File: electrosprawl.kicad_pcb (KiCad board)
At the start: 2 copper layers, 73.8 x 89.6 mm, 50 parts, among them J1 3.3v, J2 Conn_02x08_Counter_Clockwise, J3 Conn_02x06_Counter_Clockwise, J4 Conn_02x04_Counter_Clockwise, J5 Conn_02x08_Counter_Clockwise, J6 3.3v, J67 Conn_02x05_Counter_Clockwise, J7 VCC, J70 TXRX, J71 Micro_SD_Card_Det, J74 USB_B_Micro, SW1 Reset, U2 samd51p20, U5 LM1117-3.3, Y1 Crystal

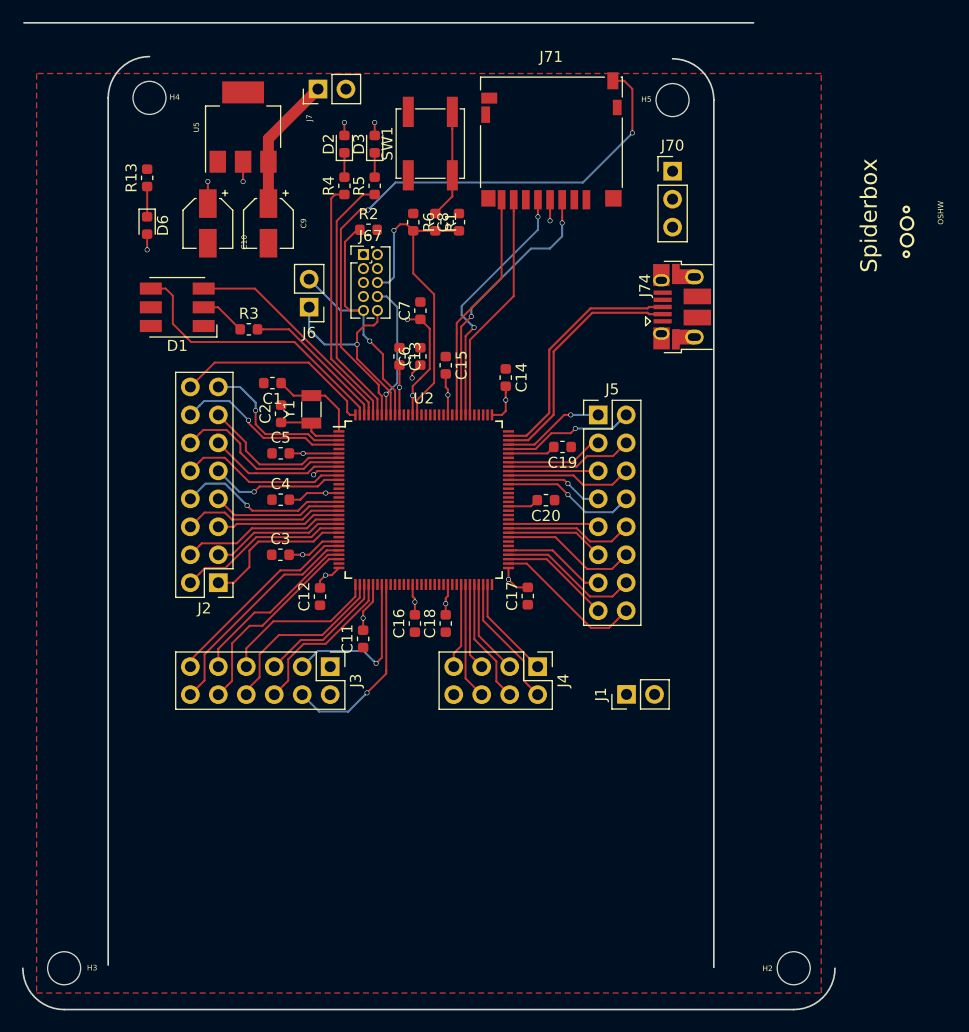
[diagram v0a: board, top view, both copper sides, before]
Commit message: update layout
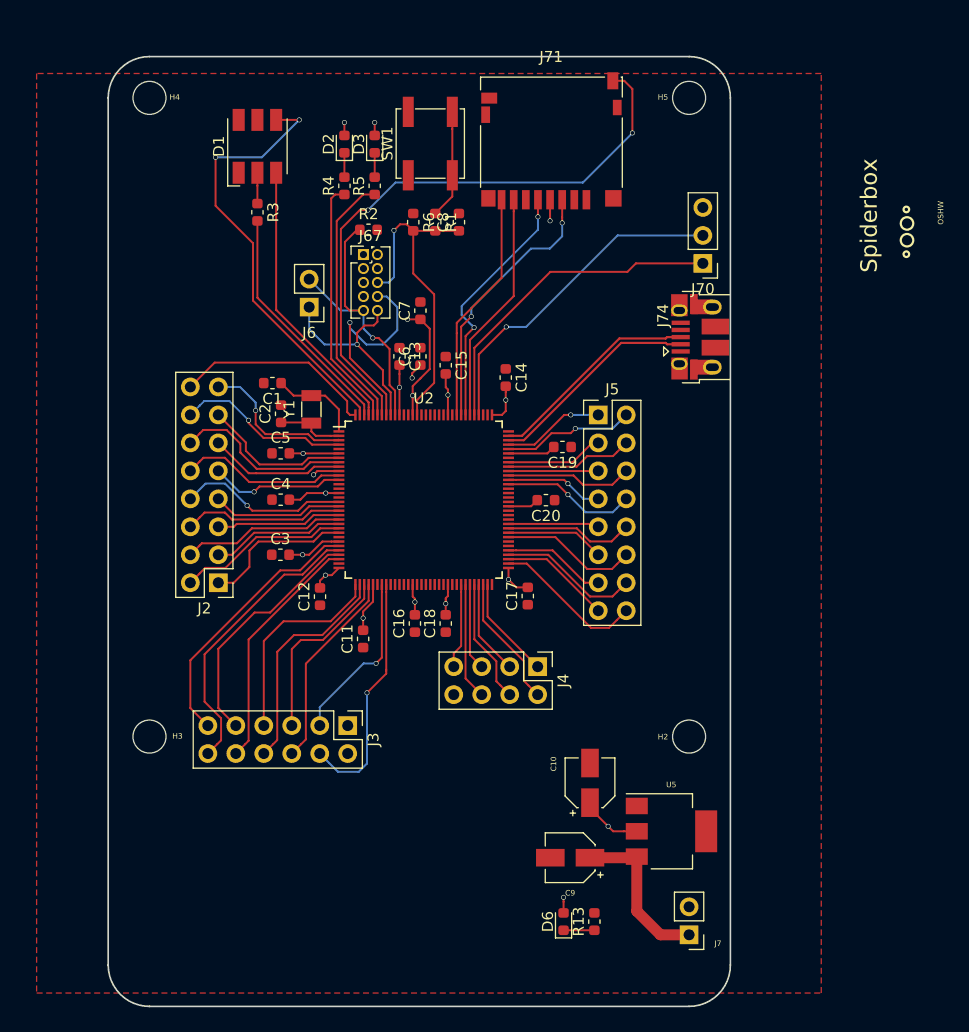
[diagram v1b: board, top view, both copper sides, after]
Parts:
- removed J1: 3.3v, Connector_PinHeader_2.54mm:PinHeader_1x02_P2.54mm_Vertical
- moved J7 83.9 mm to (161.0, 102.5), turned to 180 degrees
- moved R13 78.8 mm to (152.4, 101.3)
- moved U5 74.9 mm to (159.4, 93.1), turned to 0 degrees
- moved D6 73.7 mm to (149.6, 101.3), turned to 90 degrees
- moved C9 63.8 mm to (150.2, 95.5), turned to 180 degrees
- moved C10 61.5 mm to (152.0, 88.7), turned to 90 degrees
- moved H2 23.1 mm to (161.0, 84.5)
- moved H3 22.4 mm to (112.0, 84.5)
- moved D1 16.3 mm to (121.8, 30.9), turned to 90 degrees
- moved R3 10.7 mm to (121.8, 36.9), turned to 270 degrees
- moved J70 8.81 mm to (162.2, 41.5), turned to 180 degrees
- moved J3 5.58 mm to (130.0, 83.5)
- moved J74 3.19 mm to (162.0, 48.2)
- moved H5 1.51 mm to (161.0, 26.5)
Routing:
- net Net-(J70-Pad2): track 0.00 -> 30.3 mm, vias 0 -> 1
- net Net-(J70-Pad1): track 0.00 -> 30.0 mm
- net /D9: track 25.6 -> 40.0 mm, vias 0 -> 2
- net /D13: track 13.5 -> 21.6 mm
- net Net-(J67-Pad8): track 12.4 -> 20.0 mm
- net Net-(J3-Pad9): track 16.1 -> 22.1 mm
- net Net-(J3-Pad11): track 18.4 -> 24.4 mm
- net Net-(J3-Pad12): track 20.3 -> 26.2 mm
- net /D12: track 20.4 -> 25.5 mm
- net Net-(J3-Pad5): track 11.9 -> 16.6 mm
- net Net-(J3-Pad4): track 17.8 -> 22.3 mm
- net Net-(J3-Pad7): track 14.6 -> 18.8 mm
- net Net-(J3-Pad10): track 18.0 -> 22.1 mm
- net Net-(J3-Pad8): track 16.5 -> 20.5 mm
- net Net-(J3-Pad6): track 14.7 -> 18.2 mm
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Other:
- board size 73.8 x 89.6 mm -> 56.5 x 86.2 mm
